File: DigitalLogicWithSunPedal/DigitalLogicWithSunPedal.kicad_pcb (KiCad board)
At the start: 2 copper layers, 19 parts, among them IC1 REG1117-5, IC2 HEF4081BT,653, J1 776280-1, J2 4pin brake, J3 4pin throttle, K1 J107F1AS123VDC.36, Q1 2N2222A, U2 TS881ICT, U3 TS881ICT, U4 TS881ICT, U5 TS881ICT

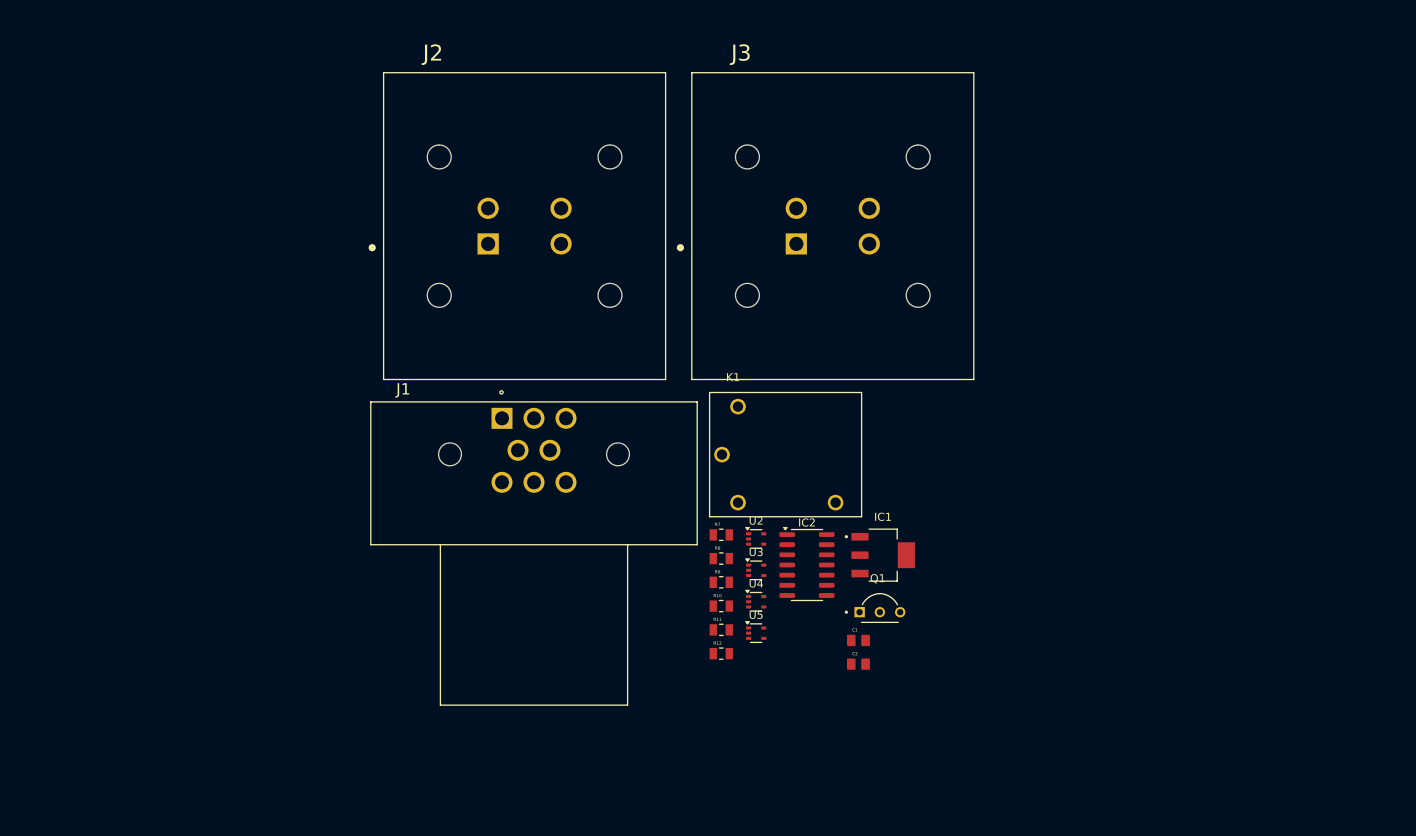
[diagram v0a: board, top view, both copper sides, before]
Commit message: Add files via upload
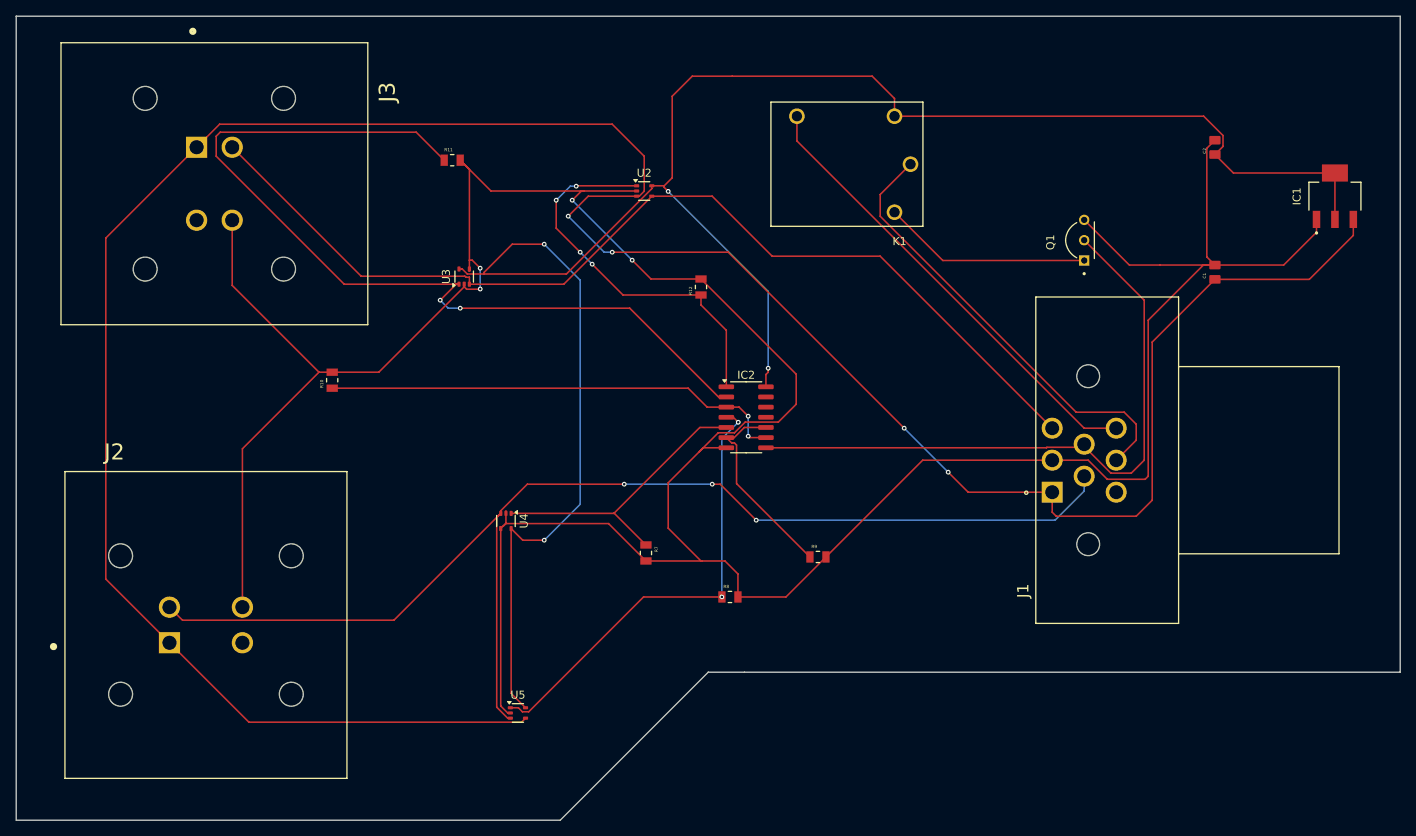
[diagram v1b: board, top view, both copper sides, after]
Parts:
- moved C2 78.5 mm to (199.8, 51.4), turned to 90 degrees
- moved J3 77.5 mm to (74.8, 55.9), turned to -90 degrees
- moved IC1 72.1 mm to (214.8, 57.5), turned to 90 degrees
- moved J1 68.8 mm to (183.5, 90.5), turned to 90 degrees
- moved R11 67.7 mm to (104.5, 53.0)
- moved C1 64.1 mm to (199.8, 67.0), turned to 90 degrees
- moved J2 63.8 mm to (73.7, 111.1)
- moved R10 56.2 mm to (89.5, 80.5), turned to 90 degrees
- moved U3 51.8 mm to (106.0, 67.5), turned to 90 degrees
- moved Q1 49.9 mm to (181.2, 63.0), turned to 90 degrees
- moved R12 45.9 mm to (135.6, 68.8), turned to 90 degrees
- moved U2 45.7 mm to (128.5, 56.9)
- moved K1 37.1 mm to (153.8, 53.5), turned to 180 degrees
- moved U4 32.9 mm to (111.2, 98.1), turned to -90 degrees
- moved U5 31.4 mm to (112.7, 122.1)
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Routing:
- net GND: track 0.00 -> 405.2 mm, vias 0 -> 4
- net +12V: track 0.00 -> 336.0 mm, vias 0 -> 4
- net +5V: track 0.00 -> 249.5 mm, vias 0 -> 4
- net Net-(U4-+): track 0.00 -> 154.2 mm, vias 0 -> 3
- net Net-(U2--): track 0.00 -> 126.7 mm
- net Net-(IC2-Pad2): track 0.00 -> 113.6 mm, vias 0 -> 2
- net Net-(IC2-Pad8): track 0.00 -> 80.4 mm
- net Net-(IC2-Pad3): track 0.00 -> 58.2 mm, vias 0 -> 2
- net Net-(J1-Pad8): track 0.00 -> 57.9 mm
- net Net-(IC2-Pad4): track 0.00 -> 57.0 mm, vias 0 -> 2
- net Net-(J1-Pad7): track 0.00 -> 56.4 mm
- net Net-(IC2-Pad1): track 0.00 -> 48.6 mm, vias 0 -> 4
- net Net-(IC2-Pad5): track 0.00 -> 37.0 mm
- net Net-(K1-PadCOIL1): track 0.00 -> 26.2 mm
- net Net-(IC2-Pad10): track 0.00 -> 24.9 mm
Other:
- board outline added: 173 x 100.5 mm
